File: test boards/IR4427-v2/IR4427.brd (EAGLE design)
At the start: 50.6 x 37 mm, 36 parts, among them IC1 IR4427, IC2 IR4427, IC3 IR4427, IC5 ACS712-LC, Q1 IRF7389, Q2 IRF7389, Q3 IRF7389

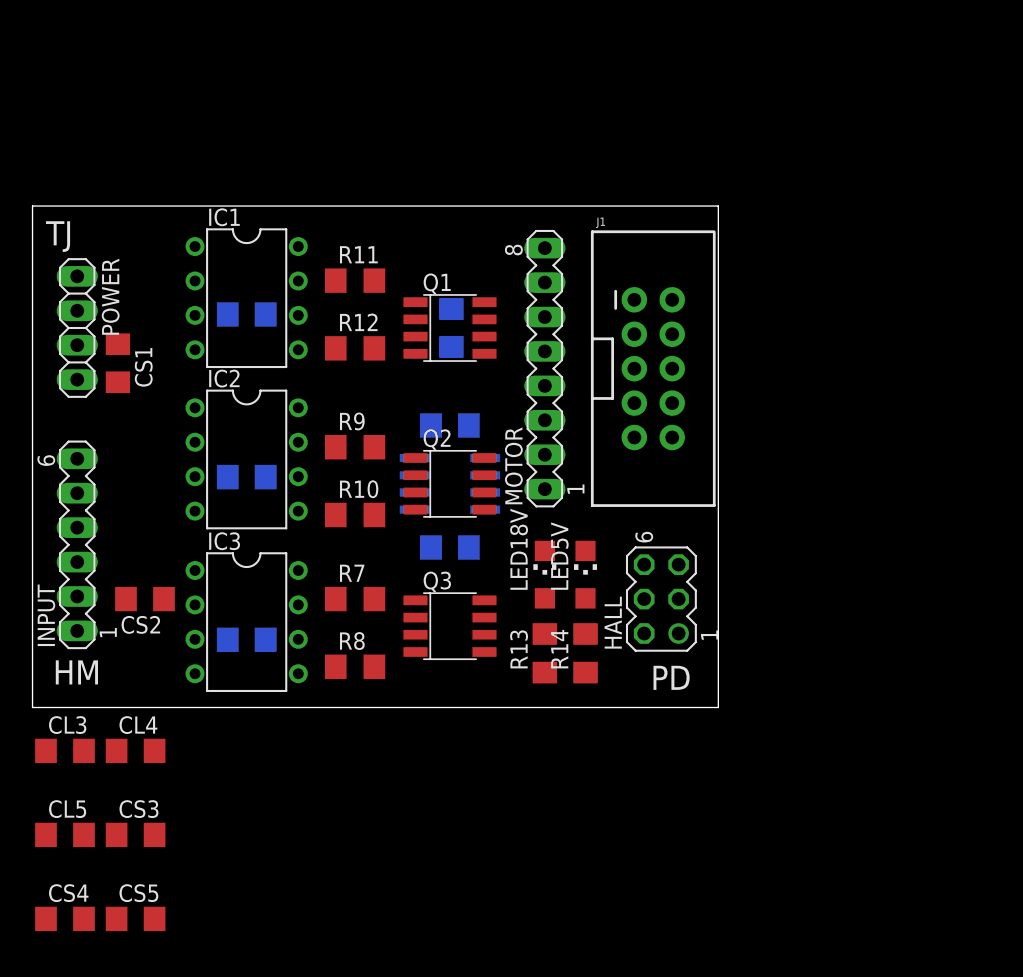
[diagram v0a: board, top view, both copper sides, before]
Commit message: Completed
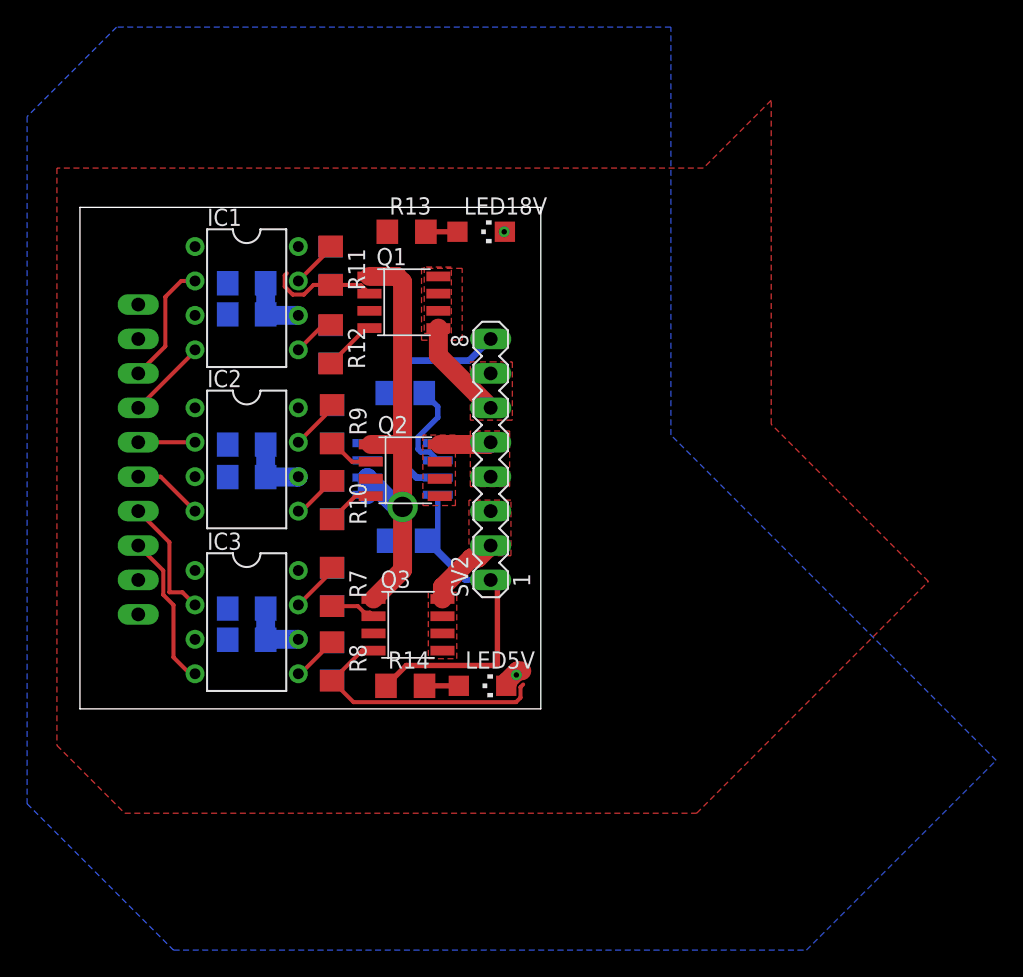
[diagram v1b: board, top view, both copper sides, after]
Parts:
- removed HALL: (no value), con-lstb:MA03-2
- removed INPUT: (no value), con-lstb:MA06-1
- removed J1: (no value), SparkFun-Connectors:2X5-SHROUDED_LOCK
- removed MOTOR: (no value), con-lstb:MA08-1
- removed POWER: (no value), pinhead:1X04
- added SV1: (no value), con-lstb:MA10-1
- added SV2: (no value), con-lstb:MA08-1
- moved CL3 40.8 mm to (32.2, 48.6), flipped to the bottom, turned to 270 degrees
- moved CS3 39.0 mm to (32.2, 42.8), flipped to the bottom, turned to 270 degrees
- moved CS4 36.6 mm to (32.3, 31.3), flipped to the bottom, turned to 270 degrees
- moved R13 32.7 mm to (37.8, 51.1), turned to 0 degrees
- moved CL4 28.1 mm to (32.3, 36.9), flipped to the bottom, turned to 270 degrees
- moved CL5 26.9 mm to (32.3, 24.9), flipped to the bottom, turned to 270 degrees
- moved LED18V 25.7 mm to (43.3, 51.1), turned to 270 degrees
- moved CS5 23.9 mm to (32.3, 19.4), flipped to the bottom, turned to 270 degrees
- moved CS 15.5 mm to (26.0, 47.3), turned to 0 degrees
- moved R14 13.5 mm to (37.7, 17.6), turned to 0 degrees
- moved CS1 11.2 mm to (26.0, 35.4), flipped to the bottom, turned to 0 degrees
- moved LED5V 11.2 mm to (43.4, 17.6), turned to 270 degrees
- moved CS2 7.53 mm to (26.0, 23.3), flipped to the bottom, turned to 0 degrees
- moved CF 4.08 mm to (37.7, 39.2)
- moved Q1 3.89 mm to (37.6, 45.9)
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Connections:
- removed net A: HALL.5, J1.6
- removed net B: HALL.3, J1.8
- removed net H1: HALL.6, MOTOR.3
- removed net H2: HALL.4, MOTOR.2
- removed net H3: HALL.2, MOTOR.1
- net 1A: now also SV1.8; no longer INPUT.6
- net 1B: now also SV1.7; no longer INPUT.5
- net 2A: now also SV1.6; no longer INPUT.4
- net 2B: now also SV1.5; no longer INPUT.3
- net 3A: now also SV1.4; no longer INPUT.2
- net 3B: now also SV1.3; no longer INPUT.1
- net ACS_OUT: now also SV2.8; no longer POWER.2
- net GND: now also SV1.1, SV1.2; no longer HALL.1, J1.3, MOTOR.4, POWER.4
- net M1: now also SV2.6, SV2.7; no longer MOTOR.8
- net M2: now also SV2.4, SV2.5; no longer MOTOR.7
- net M3: now also SV2.2, SV2.3; no longer MOTOR.6
- net VCC_18: now also SV1.10, SV1.9; no longer POWER.3
- net VCC_5V: now also SV2.1; no longer J1.2, MOTOR.5, POWER.1
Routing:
- net SINK: track 0.00 -> 34.0 mm, vias 0 -> 1
- net VCC_5V: track 0.00 -> 28.6 mm
- net 3P: track 0.00 -> 19.7 mm
- net ACS_OUT: track 0.00 -> 17.6 mm
- net VCC_18: track 0.00 -> 14.3 mm
- net 3B: track 0.00 -> 11.4 mm
- net 3A: track 0.00 -> 9.22 mm
- net 1A: track 0.00 -> 9.15 mm
- net 1N: track 0.00 -> 8.10 mm
- net M1: track 0.00 -> 7.48 mm
- net N$3: track 0.00 -> 6.95 mm
- net 1B: track 0.00 -> 6.02 mm
- net M3: track 0.00 -> 5.71 mm
- net 2B: track 0.00 -> 5.24 mm
- net 2A: track 0.00 -> 4.19 mm
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- added copper zone on layer 16, net GND
- added copper zone on layer 1, net M1
- added copper zone on layer 1, net M2
- added copper zone on layer 1, net M3
- added copper zone on layer 1, net VCC_18
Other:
- board size 50.6 x 37 mm -> 34 x 37 mm
- board text removed: "HM"
- board text removed: "KRSSG"
- board text removed: "PD"
- board text removed: "TJ"
- board text removed: "¯\_(ツ)_/¯"
